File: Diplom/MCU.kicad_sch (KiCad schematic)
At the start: 53 parts, among them IC1 E22-900T22D, J1 Conn_01x02_Pin, J2 Conn_01x05_Pin, J3 Conn_01x02_Pin, SW1 SW_Push, SW2 SW_Push, U2 BME280, U3 W25Q32JVSS, U6 STM32F411CEUx, Y3 Crystal_GND24, Y4 KX-327NHT, Y5 Crystal

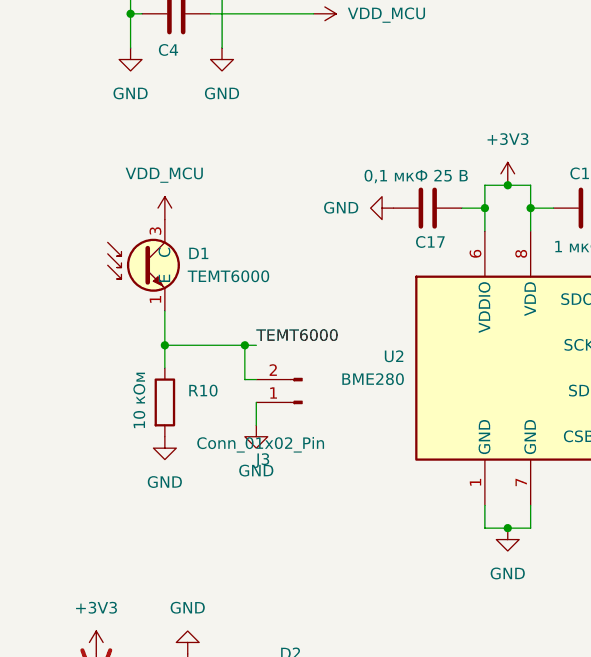
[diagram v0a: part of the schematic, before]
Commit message: corr
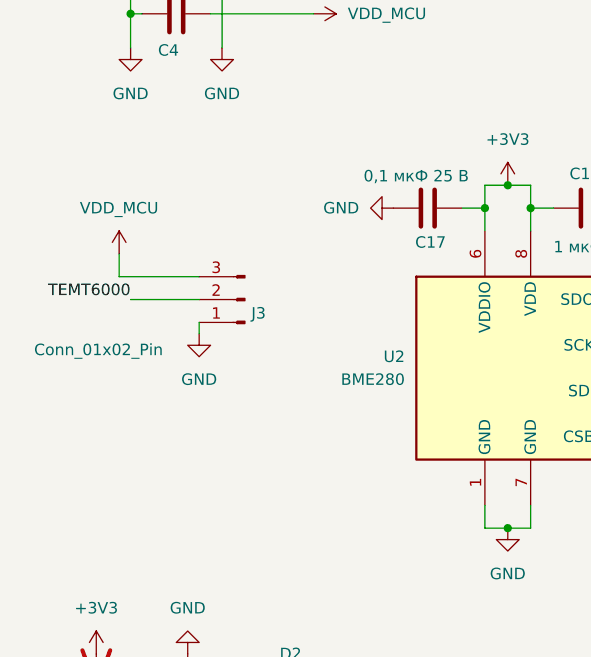
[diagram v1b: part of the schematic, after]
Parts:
- removed D1: TEMT6000, Diplom:TEMT6000, symbol Diplom:TEMT6000
- removed R10: 10 кОм, Resistor_SMD:R_0603_1608Metric_Pad0.98x0.95mm_HandSolder, symbol Device:R
- J3: footprint Connector_PinHeader_2.54mm:PinHeader_1x02_P2.54mm_Vertical -> Connector_PinHeader_2.54mm:PinHeader_1x03_P2.54mm_Vertical; symbol Connector:Conn_01x02_Pin -> Connector:Conn_01x03_Pin
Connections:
- net VDD_MCU: now also J3.3 (Pin_3)
